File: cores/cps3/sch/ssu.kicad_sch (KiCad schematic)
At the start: 1 part

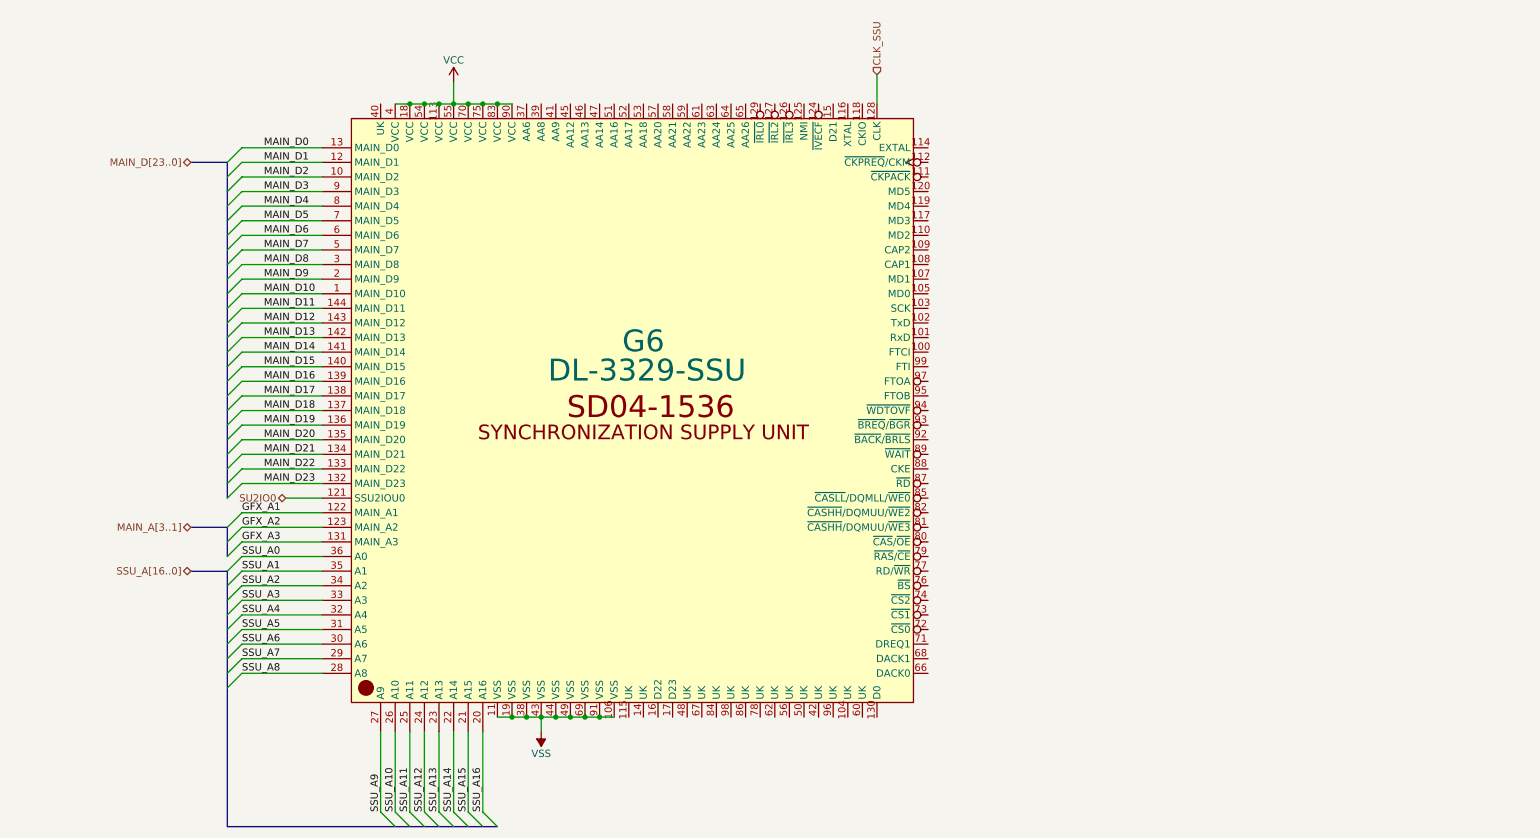
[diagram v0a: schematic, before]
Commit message: update7
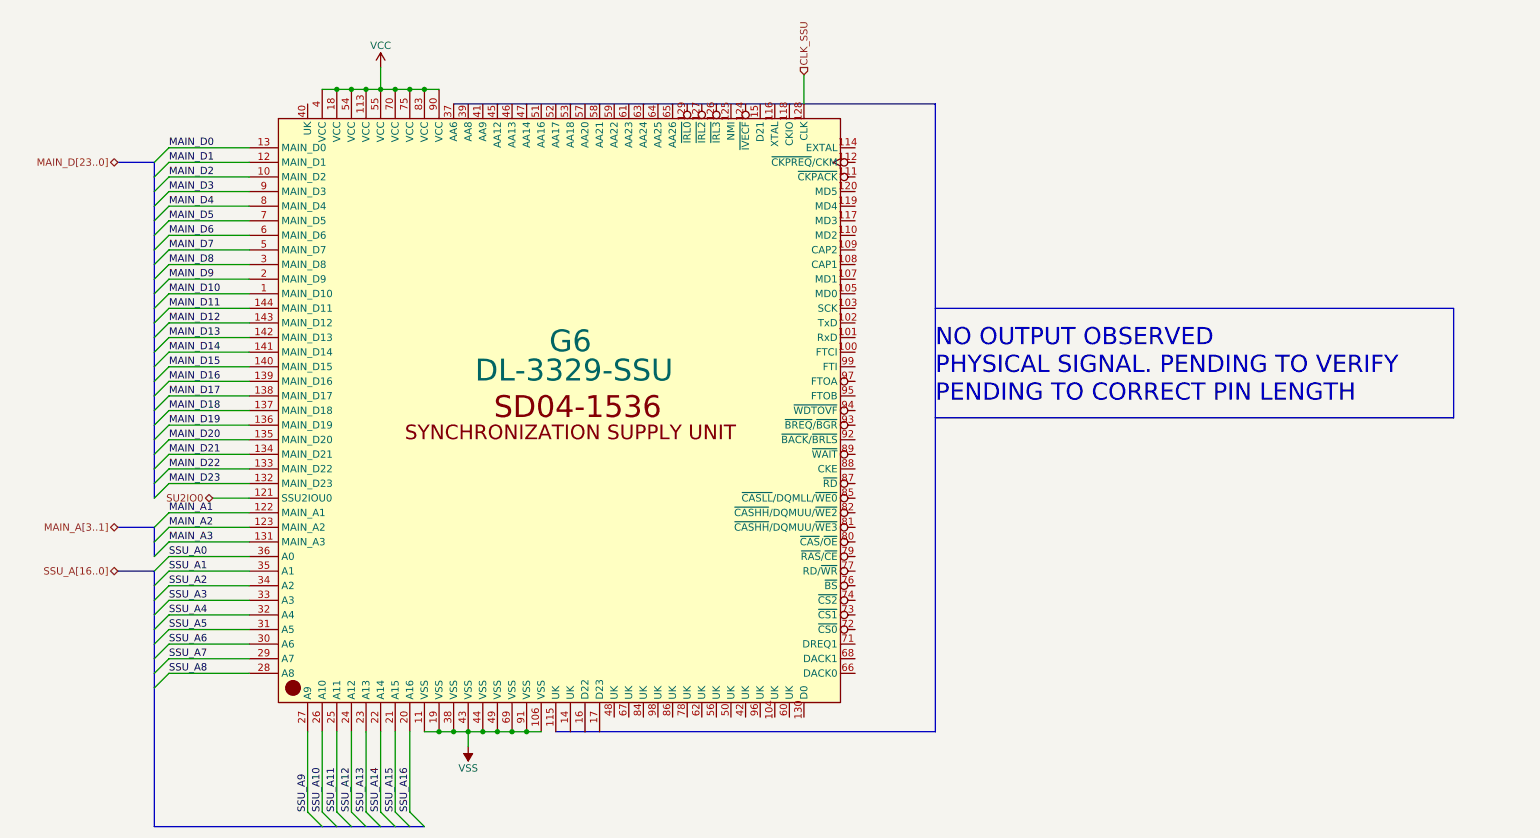
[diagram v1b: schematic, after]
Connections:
- net GFX_A1 renamed MAIN_A1
- net GFX_A2 renamed MAIN_A2
- net GFX_A3 renamed MAIN_A3
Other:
- note added: "NO OUTPUT OBSERVED PHYSICAL SIGNAL. PENDING TO VERIFY PENDING TO CORRECT PIN LENGTH"
- moved on the sheet: G6
